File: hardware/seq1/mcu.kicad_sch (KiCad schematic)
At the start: 11 parts, among them SW10 SW_Push, SW11 SW_Push, SW9 PEC12R-3220F-S0024, U5 128x64 0.96" OLED I2C

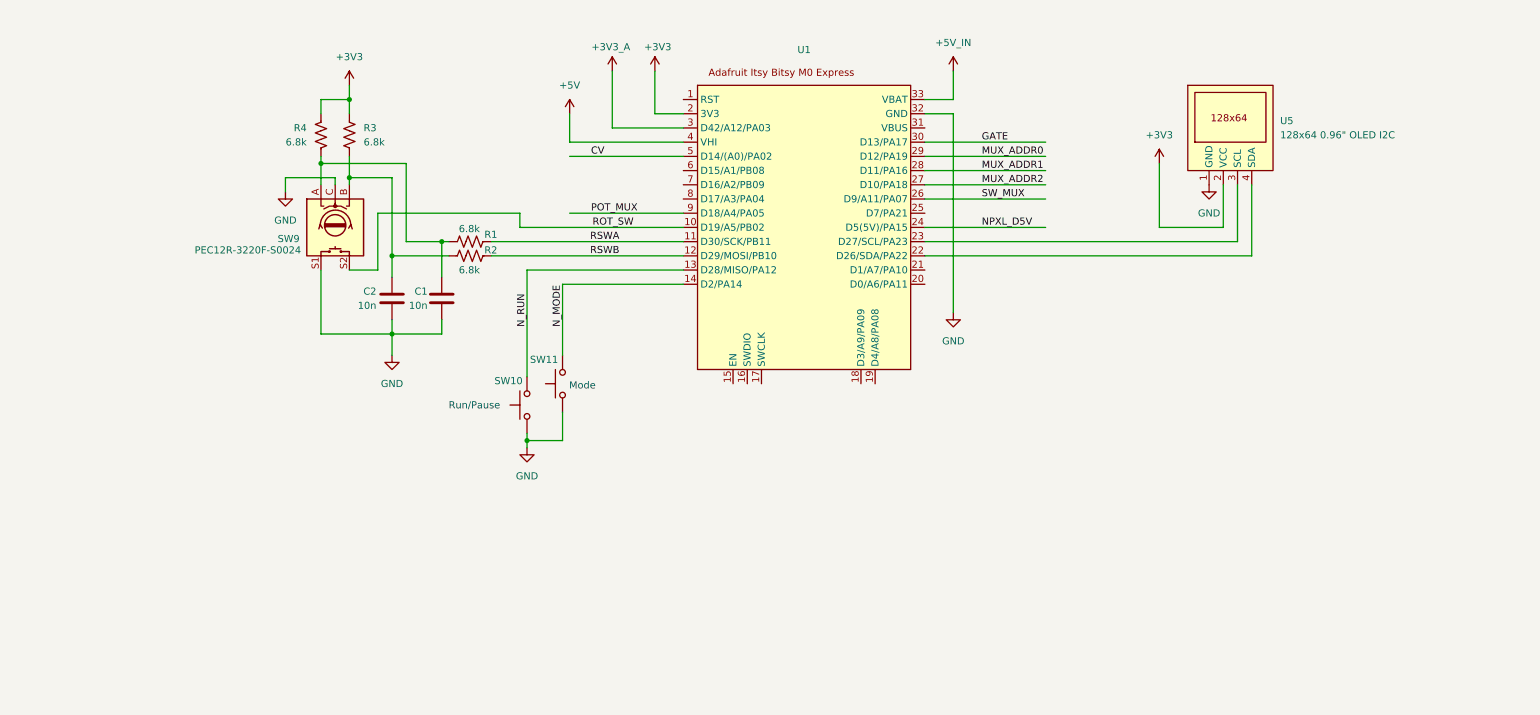
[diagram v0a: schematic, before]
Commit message: schematic and layout for v1 board
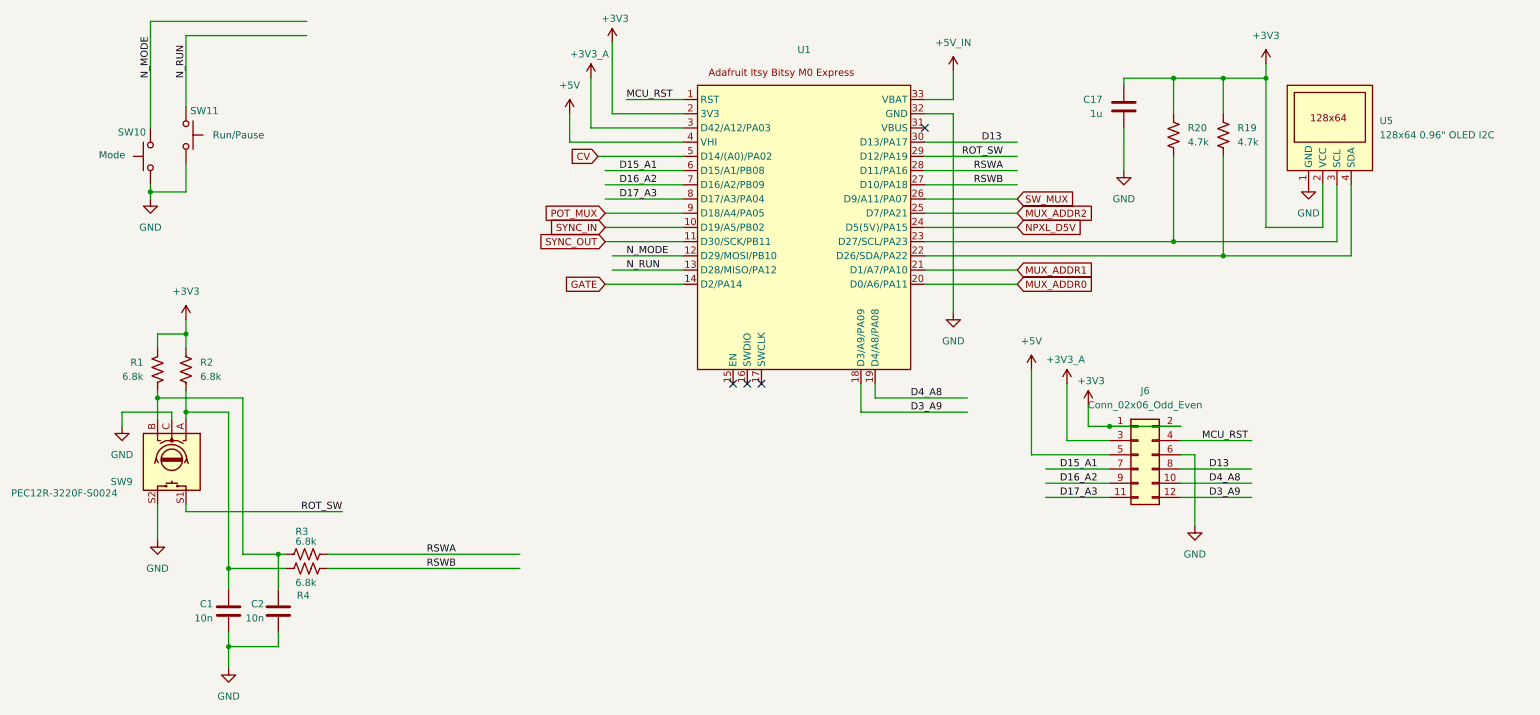
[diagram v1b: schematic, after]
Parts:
- added C17: 1u, Capacitor_THT:C_Disc_D5.0mm_W2.5mm_P5.00mm, symbol Device:C
- added J6: Conn_02x06_Odd_Even, Connector_PinHeader_2.54mm:PinHeader_2x06_P2.54mm_Vertical, symbol Connector_Generic:Conn_02x06_Odd_Even
- added R19, R20: 4.7k, Resistor_THT:R_Axial_DIN0207_L6.3mm_D2.5mm_P10.16mm_Horizontal, symbol Device:R_US
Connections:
- net +3V3: now also R1.1, R2.1, C17.1, J6.1 (Pin_1), J6.2 (Pin_2), R19.1, R20.1; no longer R3.1, R4.1
- net +3V3_A: now also J6.3 (Pin_3)
- net +5V: now also J6.5 (Pin_5)
- net GATE: now also U1.14 (D2/PA14); no longer U1.30 (D13/PA17)
- net GND: now also SW9.S2, C17.2, J6.6 (Pin_6); no longer SW9.S1
- net MUX_ADDR0: now also U1.20 (D0/A6/PA11); no longer U1.29 (D12/PA19)
- net MUX_ADDR1: now also U1.21 (D1/A7/PA10); no longer U1.28 (D11/PA16)
- net MUX_ADDR2: now also U1.25 (D7/PA21); no longer U1.27 (D10/PA18)
- net N_MODE: now also SW10.2, U1.12 (D29/MOSI/PB10); no longer SW11.2, U1.14 (D2/PA14)
- net N_RUN: now also SW11.2; no longer SW10.2
- net ROT_SW: now also SW9.S1, U1.29 (D12/PA19); no longer SW9.S2, U1.10 (D19/A5/PB02)
- net RSWA: now also R3.1, U1.28 (D11/PA16); no longer R1.1, U1.11 (D30/SCK/PB11)
- net RSWB: now also R4.1, U1.27 (D10/PA18); no longer R2.1, U1.12 (D29/MOSI/PB10)
- net MCU_RST: now reaches U1.1 (RST)
- net MCU_RST: now also J6.4 (Pin_4)
- net D3_A9: now reaches U1.18 (D3/A9/PA09)
- net D3_A9: now also J6.12 (Pin_12)
- net D4_A8: now reaches U1.19 (D4/A8/PA08)
- net D4_A8: now also J6.10 (Pin_10)
- net at U1.22 (D26/SDA/PA22), U5.4 (SDA): now also R19.2
- net at U1.23 (D27/SCL/PA23), U5.3 (SCL): now also R20.2
- net D15_A1: now reaches U1.6 (D15/A1/PB08)
- net D15_A1: now also J6.7 (Pin_7)
- net D16_A2: now reaches U1.7 (D16/A2/PB09)
- net D16_A2: now also J6.9 (Pin_9)
- net D17_A3: now reaches U1.8 (D17/A3/PA04)
- net D17_A3: now also J6.11 (Pin_11)
- net at C1.1, R4.2, SW9.A: now also R2.2; no longer R1.2
- net at C2.1, R3.2, SW9.B: now also R1.2; no longer R2.2
- new net D13: J6.8 (Pin_8), U1.30 (D13/PA17)
- new net SYNC_IN: U1.10 (D19/A5/PB02)
- new net SYNC_OUT: U1.11 (D30/SCK/PB11)
- no-connect marks 0 -> 4
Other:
- moved on the sheet: U5
